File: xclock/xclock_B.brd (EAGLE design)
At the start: 80 x 80 mm, 49 parts, among them U1 5P49V5923, U2 SI7021, U3 FIN1001, U4 FIN1001, U5 FIN1001, X1 9C-24.000MEEJ-T

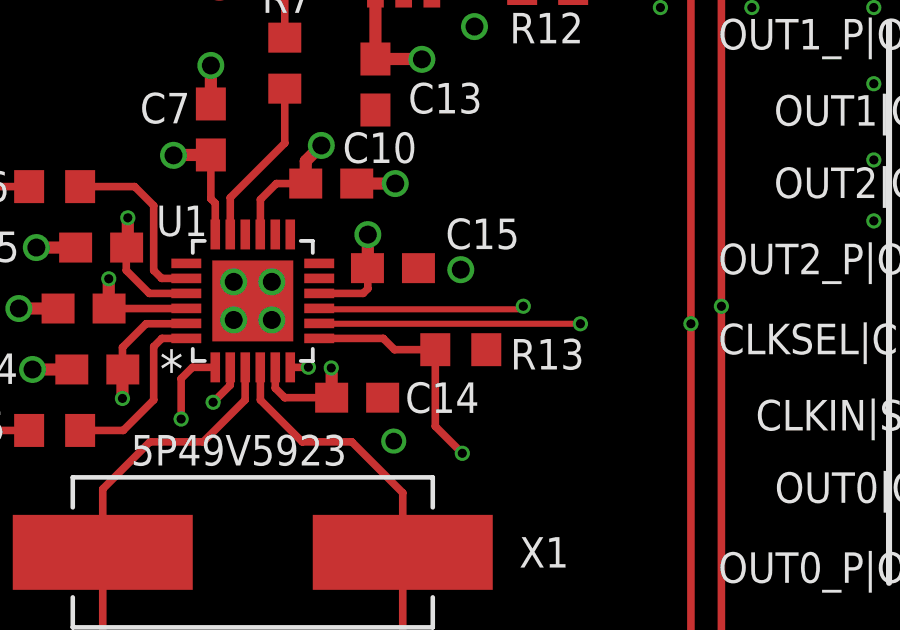
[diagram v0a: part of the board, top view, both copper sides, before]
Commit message: xclock: final tweaks
Signed-off-by: malo <pavol.malosek@gmail.com>
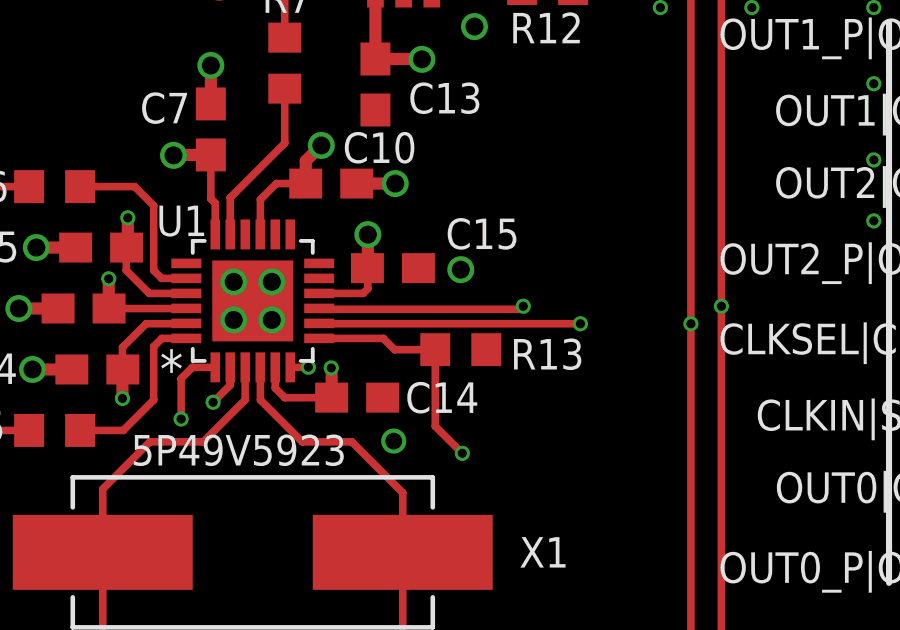
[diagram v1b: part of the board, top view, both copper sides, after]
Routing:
- net VDDA: track 17.7 -> 17.1 mm
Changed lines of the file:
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@@
 <setting verticaltext="up"/>
 </settings>
-<grid distance="1" unitdist="mil" unit="mil" style="lines" multiple="1" display="yes" altdistance="0.025" altunitdist="inch" altunit="inch"/>
+<grid distance="5" unitdist="mil" unit="mil" style="lines" multiple="1" display="yes" altdistance="0.025" altunitdist="inch" altunit="inch"/>
 <layers>
 <layer number="1" name="Top" color="4" fill="1" visible="yes" active="yes"/>
@@
 <layer number="42" name="bRestrict" color="1" fill="10" visible="yes" active="yes"/>
 <layer number="43" name="vRestrict" color="2" fill="10" visible="yes" active="yes"/>
-<layer number="44" name="Drills" color="7" fill="1" visible="no" active="yes"/>
+<layer number="44" name="Drills" color="7" fill="1" visible="yes" active="yes"/>
 <layer number="45" name="Holes" color="7" fill="1" visible="yes" active="yes"/>
 <layer number="46" name="Milling" color="3" fill="1" visible="yes" active="yes"/>
@@
 <contactref element="U$1" pad="113"/>
 <wire x1="46.538" y1="39.255" x2="46.55" y2="39.243" width="0.254" layer="1"/>
-<wire x1="46.55" y1="39.243" x2="55.245" y2="39.243" width="0.2032" layer="1"/>
+<wire x1="46.55" y1="39.243" x2="55.245" y2="39.243" width="0.254" layer="1"/>
 <via x="55.245" y="39.243" extent="1-16" drill="0.3048"/>
 <wire x1="55.245" y1="39.243" x2="58.928" y2="39.243" width="0.254" layer="2"/>
@@
 <contactref element="U$1" pad="114"/>
 <wire x1="46.538" y1="39.755" x2="46.5674" y2="39.7256" width="0.254" layer="1"/>
-<wire x1="46.5674" y1="39.7256" x2="53.2384" y2="39.7256" width="0.2032" layer="1"/>
-<wire x1="53.2384" y1="39.7256" x2="53.34" y2="39.8272" width="0.2032" layer="1"/>
+<wire x1="46.5674" y1="39.7256" x2="53.2384" y2="39.7256" width="0.254" layer="1"/>
+<wire x1="53.2384" y1="39.7256" x2="53.34" y2="39.8272" width="0.254" layer="1"/>
 <via x="53.34" y="39.8272" extent="1-16" drill="0.3048"/>
 <wire x1="53.34" y1="39.8272" x2="59.944" y2="39.8272" width="0.254" layer="2"/>
@@
 <wire x1="48.1584" y1="41.3766" x2="48.1584" y2="42.2148" width="0.4064" layer="1"/>
 <via x="48.1584" y="42.2148" extent="1-16" drill="0.6" shape="square"/>
-<wire x1="48.1584" y1="42.2148" x2="48.6918" y2="42.3164" width="0.4064" layer="15"/>
 <contactref element="VDDA" pad="1"/>
 </signal>
@@
 <wire x1="36.2966" y1="22.1742" x2="61.3156" y2="22.1742" width="0.254" layer="2"/>
 <wire x1="35.433" y1="35.687" x2="35.433" y2="34.9758" width="0.254" layer="1"/>
-<via x="35.433" y="34.9758" extent="1-16" drill="0.3048" shape="square"/>
+<via x="35.433" y="34.9758" extent="1-16" drill="0.3048"/>
 <wire x1="35.433" y1="34.9758" x2="35.433" y2="23.0378" width="0.254" layer="2"/>
 <wire x1="61.3156" y1="22.1742" x2="63.9572" y2="24.8158" width="0.254" layer="2"/>
@@
 <via x="35.4076" y="44.6024" extent="1-16" drill="0.3048"/>
 <wire x1="35.4076" y1="44.6024" x2="35.4076" y2="55.4482" width="0.254" layer="2"/>
-<wire x1="63.7286" y1="56.007" x2="67.31" y2="56.007" width="0.2032" layer="2"/>
-<wire x1="67.31" y1="56.007" x2="69.8754" y2="53.4416" width="0.2032" layer="2"/>
-<wire x1="69.8754" y1="53.4416" x2="69.8754" y2="48.6664" width="0.2032" layer="2"/>
-<wire x1="69.8754" y1="48.6664" x2="70.8914" y2="47.6504" width="0.2032" layer="2"/>
-<wire x1="70.8914" y1="47.6504" x2="72.39" y2="47.6504" width="0.2032" layer="2"/>
-<wire x1="72.39" y1="47.6504" x2="76.1746" y2="47.6504" width="0.2032" layer="2"/>
-<wire x1="76.1746" y1="47.6504" x2="77.47" y2="46.355" width="0.2032" layer="2"/>
-<wire x1="72.39" y1="46.355" x2="72.39" y2="47.6504" width="0.2032" layer="2"/>
+<wire x1="63.7286" y1="56.007" x2="67.31" y2="56.007" width="0.254" layer="2"/>
+<wire x1="67.31" y1="56.007" x2="69.8754" y2="53.4416" width="0.254" layer="2"/>
+<wire x1="69.8754" y1="53.4416" x2="69.8754" y2="48.6664" width="0.254" layer="2"/>
+<wire x1="69.8754" y1="48.6664" x2="70.8914" y2="47.6504" width="0.254" layer="2"/>
+<wire x1="70.8914" y1="47.6504" x2="72.39" y2="47.6504" width="0.254" layer="2"/>
+<wire x1="72.39" y1="47.6504" x2="76.1746" y2="47.6504" width="0.254" layer="2"/>
+<wire x1="76.1746" y1="47.6504" x2="77.47" y2="46.355" width="0.254" layer="2"/>
+<wire x1="72.39" y1="46.355" x2="72.39" y2="47.6504" width="0.254" layer="2"/>
 </signal>
 <signal name="OUT2">
@@
 <via x="48.4124" y="54.5592" extent="1-16" drill="0.3048"/>
 <wire x1="48.4124" y1="54.5592" x2="48.4124" y2="53.0098" width="0.254" layer="1"/>
-<wire x1="65.2272" y1="54.5592" x2="65.4812" y2="54.5592" width="0.2032" layer="2"/>
-<wire x1="65.4812" y1="54.5592" x2="68.4276" y2="51.6128" width="0.2032" layer="2"/>
-<wire x1="68.4276" y1="51.6128" x2="68.4276" y2="46.5074" width="0.2032" layer="2"/>
-<wire x1="68.4276" y1="46.5074" x2="69.8246" y2="45.1104" width="0.2032" layer="2"/>
-<wire x1="69.8246" y1="45.1104" x2="72.39" y2="45.1104" width="0.2032" layer="2"/>
-<wire x1="72.39" y1="45.1104" x2="76.1746" y2="45.1104" width="0.2032" layer="2"/>
-<wire x1="76.1746" y1="45.1104" x2="77.47" y2="43.815" width="0.2032" layer="2"/>
-<wire x1="72.39" y1="43.815" x2="72.39" y2="45.1104" width="0.2032" layer="2"/>
+<wire x1="65.2272" y1="54.5592" x2="65.4812" y2="54.5592" width="0.254" layer="2"/>
+<wire x1="65.4812" y1="54.5592" x2="68.4276" y2="51.6128" width="0.254" layer="2"/>
+<wire x1="68.4276" y1="51.6128" x2="68.4276" y2="46.5074" width="0.254" layer="2"/>
+<wire x1="68.4276" y1="46.5074" x2="69.8246" y2="45.1104" width="0.254" layer="2"/>
+<wire x1="69.8246" y1="45.1104" x2="72.39" y2="45.1104" width="0.254" layer="2"/>
+<wire x1="72.39" y1="45.1104" x2="76.1746" y2="45.1104" width="0.254" layer="2"/>
+<wire x1="76.1746" y1="45.1104" x2="77.47" y2="43.815" width="0.254" layer="2"/>
+<wire x1="72.39" y1="43.815" x2="72.39" y2="45.1104" width="0.254" layer="2"/>
 </signal>
 <signal name="VDDD">
@@
 <wire x1="71.39143125" y1="57.4548" x2="74.676" y2="54.17023125" width="0.254" layer="2"/>
 <wire x1="74.676" y1="54.17023125" x2="74.676" y2="52.9844" width="0.254" layer="2"/>
-<wire x1="74.676" y1="52.9844" x2="72.39" y2="50.6984" width="0.2032" layer="2"/>
-<wire x1="72.39" y1="50.6984" x2="72.39" y2="48.895" width="0.2032" layer="2"/>
+<wire x1="74.676" y1="52.9844" x2="72.39" y2="50.6984" width="0.254" layer="2"/>
+<wire x1="72.39" y1="50.6984" x2="72.39" y2="48.895" width="0.254" layer="2"/>
 </signal>
 <signal name="OUT2_P">
@@
 <wire x1="42.3112" y1="37.79" x2="41.9354" y2="37.4142" width="0.254" layer="1"/>
 <wire x1="41.9354" y1="37.4142" x2="41.9354" y2="36.068" width="0.254" layer="1"/>
-<via x="41.9354" y="36.068" extent="1-16" drill="0.3048" shape="square"/>
+<via x="41.9354" y="36.068" extent="1-16" drill="0.3048"/>
 <wire x1="41.9354" y1="36.068" x2="72.263" y2="36.068" width="0.254" layer="2"/>
 <contactref element="J1" pad="16"/>
@@
 <wire x1="43.573" y1="37.79" x2="43.573" y2="37.1976" width="0.254" layer="1"/>
 <wire x1="43.573" y1="37.1976" x2="43.0022" y2="36.6268" width="0.254" layer="1"/>
-<via x="43.0022" y="36.6268" extent="1-16" drill="0.3048" shape="square"/>
+<via x="43.0022" y="36.6268" extent="1-16" drill="0.3048"/>
 <wire x1="43.0022" y1="36.6268" x2="68.5292" y2="36.6268" width="0.254" layer="2"/>
 <contactref element="J1" pad="15"/>
@@
 <wire x1="50.4072" y1="38.3794" x2="50.4072" y2="35.8258" width="0.254" layer="1"/>
 <wire x1="50.4072" y1="35.8258" x2="51.308" y2="34.925" width="0.254" layer="1"/>
-<via x="51.308" y="34.925" extent="1-16" drill="0.3048" shape="square"/>
+<via x="51.308" y="34.925" extent="1-16" drill="0.3048"/>
 <wire x1="51.308" y1="34.925" x2="76.2" y2="34.925" width="0.254" layer="2"/>
 <wire x1="76.2" y1="34.925" x2="77.47" y2="36.195" width="0.254" layer="2"/>
@@
 <wire x1="74.7776" y1="20.22636875" x2="74.7776" y2="27.8892" width="0.254" layer="2"/>
 <wire x1="74.7776" y1="27.8892" x2="72.39" y2="30.2768" width="0.254" layer="2"/>
-<wire x1="72.39" y1="30.2768" x2="72.39" y2="31.115" width="0.2032" layer="2"/>
+<wire x1="72.39" y1="30.2768" x2="72.39" y2="31.115" width="0.254" layer="2"/>
 </signal>
 <signal name="OUT0_N">
@@
 <contactref element="J1" pad="24"/>
 <wire x1="19.8374" y1="37.2618" x2="19.8374" y2="37.9476" width="0.254" layer="1"/>
-<via x="19.8374" y="37.9476" extent="1-16" drill="0.3048" shape="square"/>
-<wire x1="19.8374" y1="37.9476" x2="19.8374" y2="34.8996" width="0.254" layer="2"/>
-<wire x1="19.8374" y1="34.8996" x2="20.1422" y2="34.5948" width="0.254" layer="2"/>
-<wire x1="20.1422" y1="34.5948" x2="20.1422" y2="16.53795" width="0.254" layer="2"/>
+<via x="19.8374" y="37.9476" extent="1-16" drill="0.3048"/>
+<wire x1="19.8374" y1="37.9476" x2="20.1422" y2="37.6428" width="0.254" layer="2"/>
+<wire x1="20.1422" y1="37.6428" x2="20.1422" y2="16.53795" width="0.254" layer="2"/>
 <wire x1="20.1422" y1="16.53795" x2="21.82115" y2="14.859" width="0.254" layer="2"/>
 <wire x1="21.82115" y1="14.859" x2="69.98496875" y2="14.859" width="0.254" layer="2"/>

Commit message: xclock: update with recent library changes + xtal cap values updated to 15p
Signed-off-by: malo <pavol.malosek@gmail.com>
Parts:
- C1, C2: value (none) -> 15p
- R10, R11, R12, R3, R4, R9: value 33 -> 0
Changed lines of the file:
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@@
 </autorouter>
 <elements>
-<element name="C1" library="rcl" package="C0603" value="" x="38.481" y="27.686" smashed="yes">
+<element name="C1" library="rcl" package="C0603" value="15p" x="38.481" y="27.686" smashed="yes">
 <attribute name="NAME" x="39.37" y="26.797" size="1.016" layer="25" font="vector" ratio="15" rot="R180"/>
-<attribute name="VALUE" x="37.846" y="25.781" size="1.27" layer="27"/>
 </element>
 <element name="C10" library="rcl" package="C0603" value="0.1u" x="46.9392" y="43.9166" smashed="yes" rot="R180">
 <attribute name="NAME" x="47.3202" y="44.6024" size="1.016" layer="25" font="vector" ratio="15"/>
 </element>
-<element name="C2" library="rcl" package="C0603" value="" x="50.165" y="27.686" smashed="yes" rot="R180">
+<element name="C2" library="rcl" package="C0603" value="15p" x="50.165" y="27.686" smashed="yes" rot="R180">
 <attribute name="NAME" x="51.054" y="26.797" size="1.016" layer="25" font="vector" ratio="15" rot="R180"/>
-<attribute name="VALUE" x="50.8" y="29.591" size="1.27" layer="27" rot="R180"/>
 </element>
 <element name="C4" library="rcl" package="C0603" value="0.1u" x="39.1414" y="37.719" smashed="yes">
@@
 <attribute name="NAME" x="49.5046" y="46.2534" size="1.016" layer="25" font="vector" ratio="15"/>
 </element>
-<element name="R3" library="rcl" package="R0603" value="33" x="24.2062" y="35.7124" smashed="yes">
+<element name="R3" library="rcl" package="R0603" value="0" x="24.2062" y="35.7124" smashed="yes">
 <attribute name="NAME" x="23.5966" y="36.449" size="1.016" layer="25" font="vector" ratio="15"/>
 </element>
-<element name="R4" library="rcl" package="R0603" value="33" x="24.2062" y="38.3032" smashed="yes">
+<element name="R4" library="rcl" package="R0603" value="0" x="24.2062" y="38.3032" smashed="yes">
 <attribute name="NAME" x="23.5966" y="39.116" size="1.016" layer="25" font="vector" ratio="15"/>
 </element>
-<element name="R9" library="rcl" package="R0603" value="33" x="24.2062" y="43.815" smashed="yes">
+<element name="R9" library="rcl" package="R0603" value="0" x="24.2062" y="43.815" smashed="yes">
 <attribute name="NAME" x="23.495" y="44.577" size="1.016" layer="25" font="vector" ratio="15"/>
 </element>
-<element name="R10" library="rcl" package="R0603" value="33" x="24.2062" y="46.3804" smashed="yes">
+<element name="R10" library="rcl" package="R0603" value="0" x="24.2062" y="46.3804" smashed="yes">
 <attribute name="NAME" x="22.987" y="47.244" size="1.016" layer="25" font="vector" ratio="15"/>
 </element>
-<element name="R11" library="rcl" package="R0603" value="33" x="54.1528" y="53.0098" smashed="yes" rot="R180">
+<element name="R11" library="rcl" package="R0603" value="0" x="54.1528" y="53.0098" smashed="yes" rot="R180">
 <attribute name="NAME" x="52.9082" y="53.8226" size="1.016" layer="25" font="vector" ratio="15"/>
 </element>
-<element name="R12" library="rcl" package="R0603" value="33" x="54.1528" y="50.419" smashed="yes" rot="R180">
+<element name="R12" library="rcl" package="R0603" value="0" x="54.1528" y="50.419" smashed="yes" rot="R180">
 <attribute name="NAME" x="52.8828" y="48.5902" size="1.016" layer="25" font="vector" ratio="15"/>
 </element>
